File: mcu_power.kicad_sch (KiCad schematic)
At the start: 1 part, among them U1 STM32H743ZITx

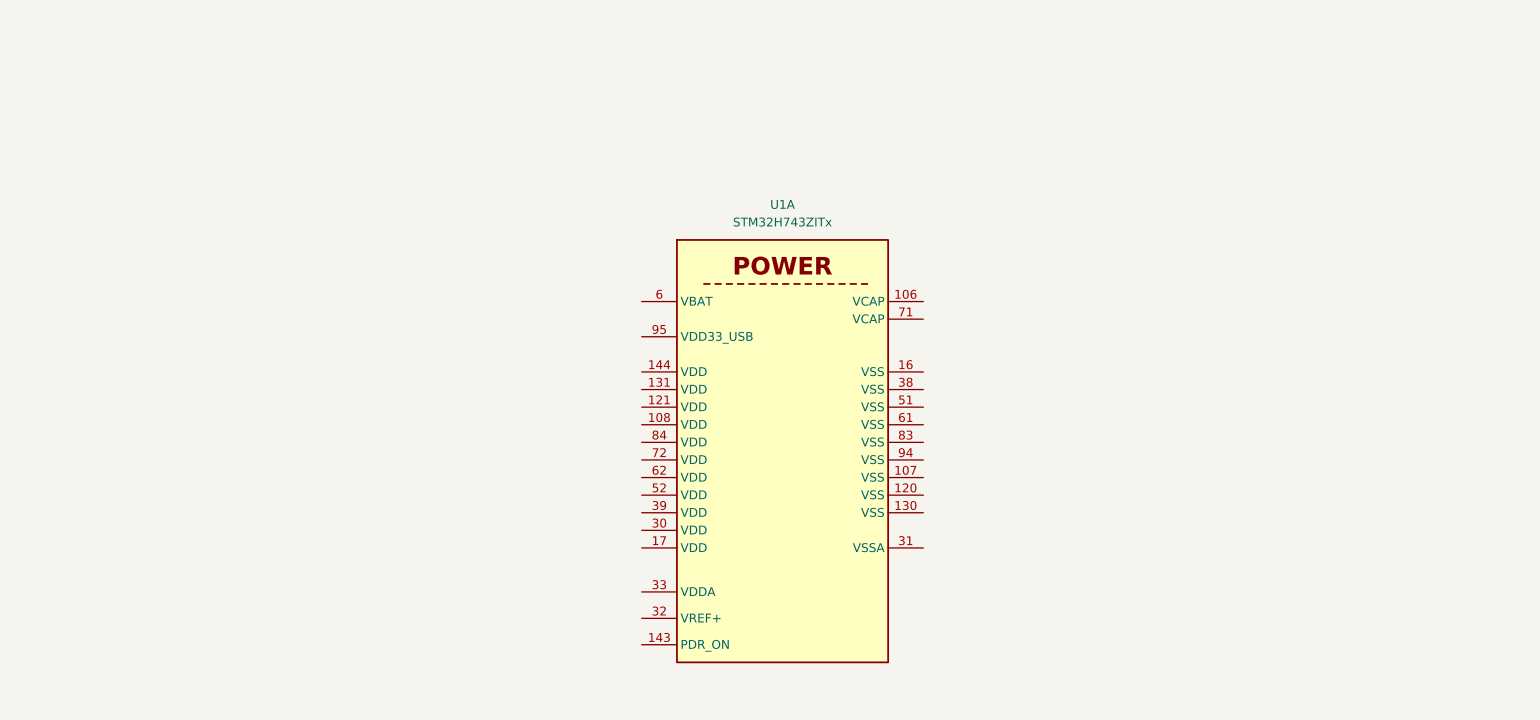
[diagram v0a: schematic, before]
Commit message: more passives work
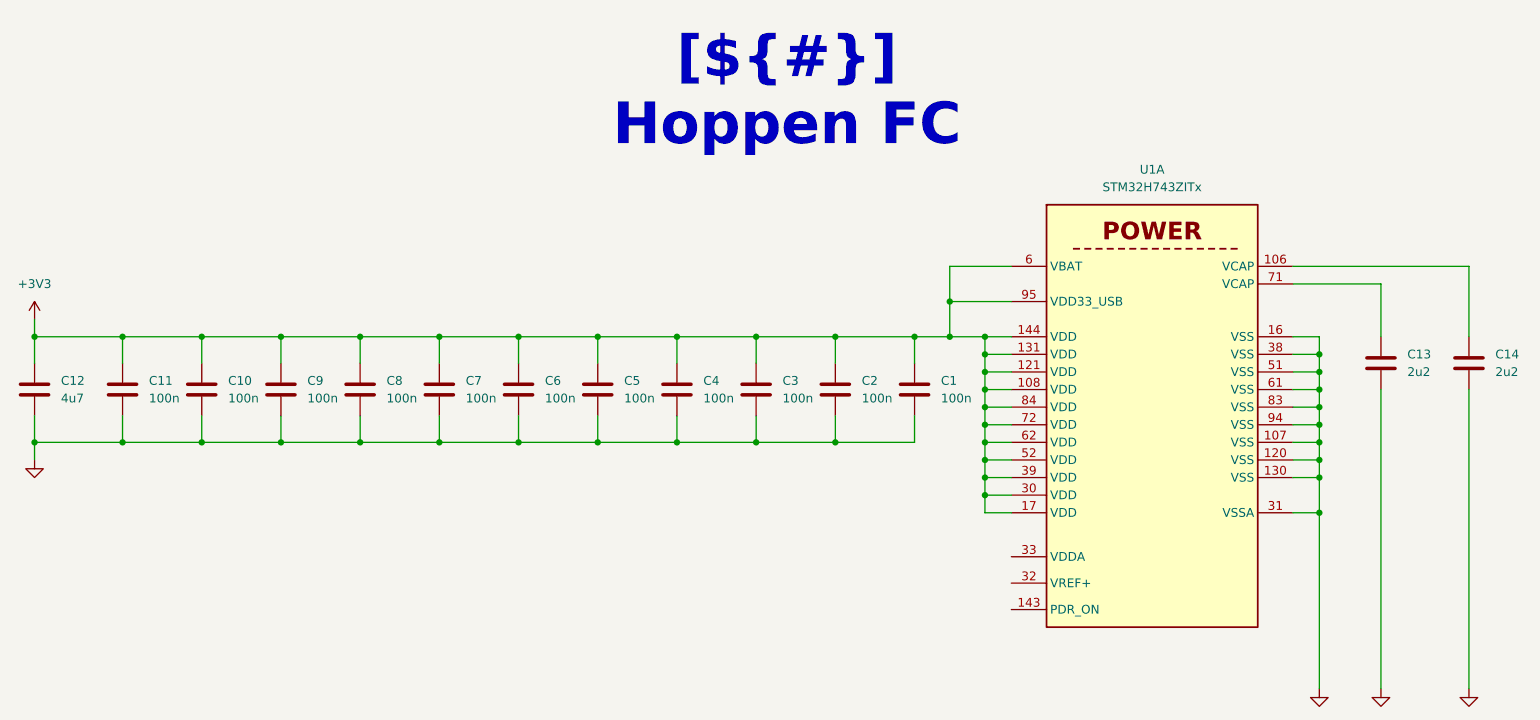
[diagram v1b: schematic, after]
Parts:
- added C1, C10, C11, C2, C3, C4, C5, C6, C7, C8, C9: 100n, 0_capacitor_smd:C_0402_1005Metric, symbol Device:C
- added C12: 4u7, 0_capacitor_smd:C_0603_1608Metric, symbol Device:C
- added C13, C14: 2u2, 0_capacitor_smd:C_0603_1608Metric, symbol Device:C
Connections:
- net at U1.106 (VCAP): now also C14.1
- net GND: now reaches U1.107 (VSS)
- net GND: now also U1.120 (VSS), U1.130 (VSS), U1.16 (VSS), U1.31 (VSSA), U1.38 (VSS), U1.51 (VSS), U1.61 (VSS), U1.83 (VSS), U1.94 (VSS), C1.2, C10.2, C11.2, C12.2, C13.2, C14.2, C2.2, C3.2, C4.2, C5.2, C6.2, C7.2, C8.2, C9.2
- net +3V3: now reaches U1.108 (VDD)
- net +3V3: now also U1.121 (VDD), U1.131 (VDD), U1.144 (VDD), U1.17 (VDD), U1.30 (VDD), U1.39 (VDD), U1.52 (VDD), U1.6 (VBAT), U1.62 (VDD), U1.72 (VDD), U1.84 (VDD), U1.95 (VDD33_USB), C1.1, C10.1, C11.1, C12.1, C2.1, C3.1, C4.1, C5.1, C6.1, C7.1, C8.1, C9.1
- net at U1.71 (VCAP): now also C13.1
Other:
- moved on the sheet: U1A
